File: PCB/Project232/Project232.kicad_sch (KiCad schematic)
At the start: 28 parts, among them J1 BOOT MODE, J2 USB_B_Micro, J3 SW, SW1 RESET, U1 STM32F103C8Tx, U2 AMS1117-3.3

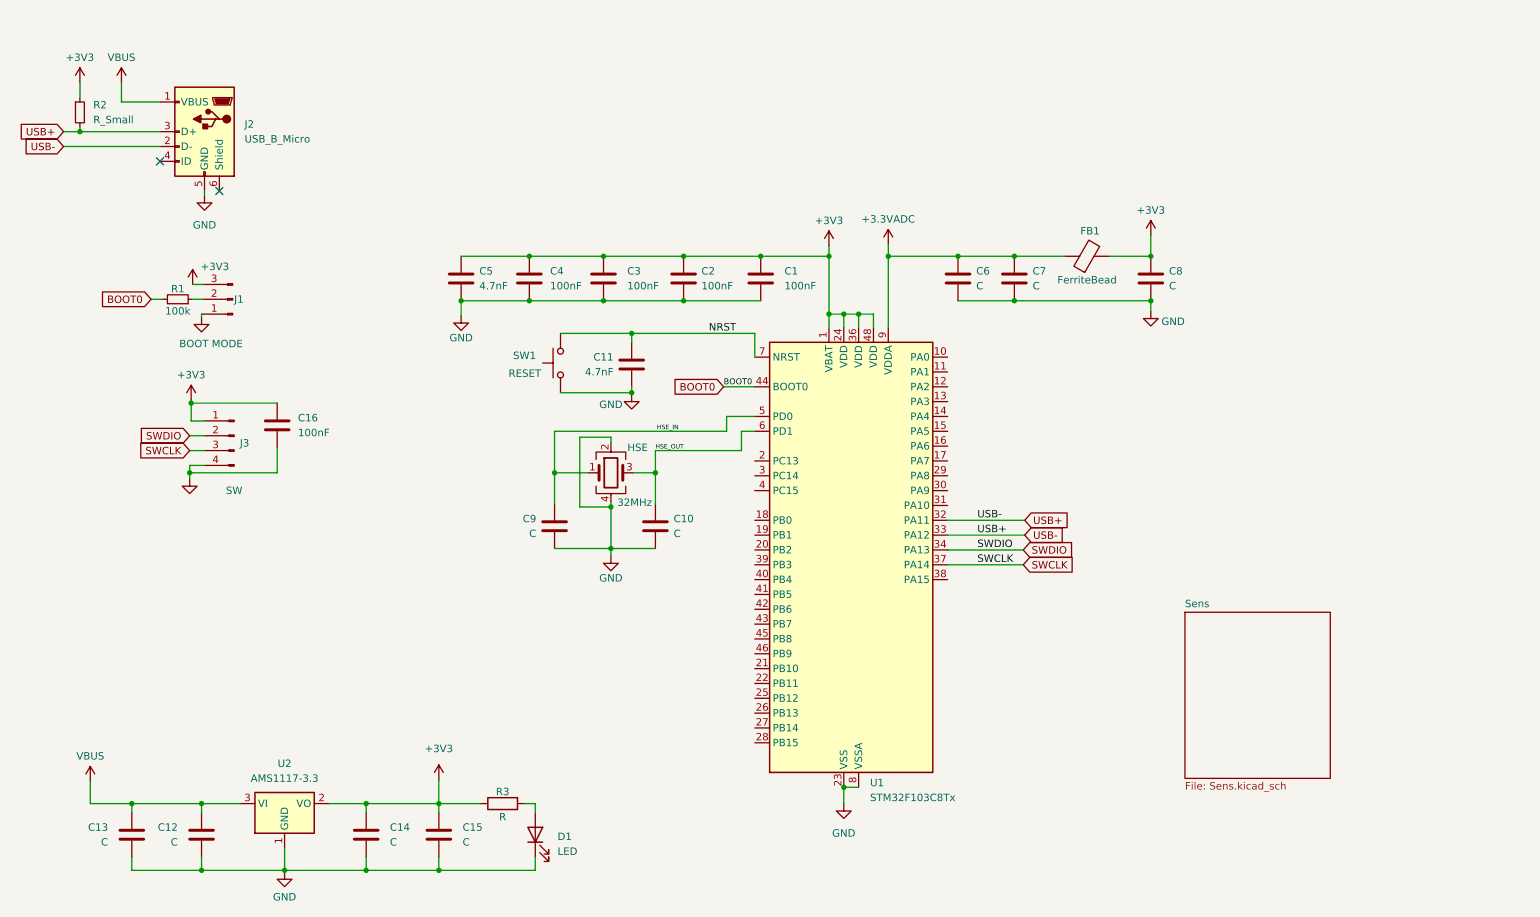
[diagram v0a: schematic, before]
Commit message: update test board and docs
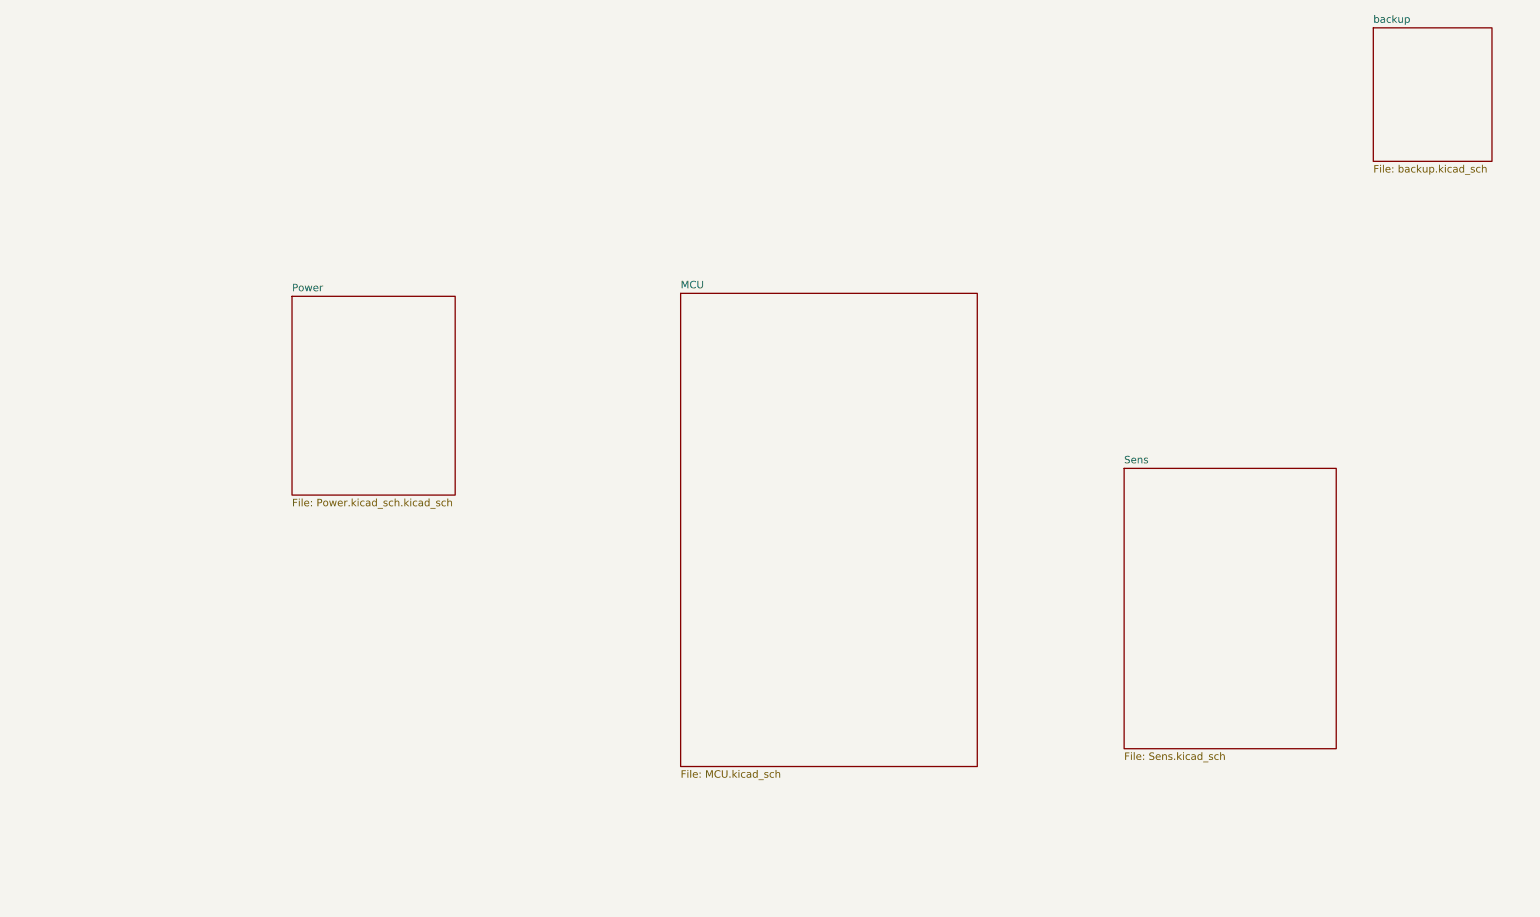
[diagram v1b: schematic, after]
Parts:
- removed C1, C16, C2, C3, C4: 100nF, symbol Device:C
- removed C10, C12, C13, C14, C15, C6, C7, C8, C9: C, symbol Device:C
- removed C11, C5: 4.7nF, symbol Device:C
- removed D1: LED, symbol Device:LED
- removed FB1: FerriteBead, symbol Device:FerriteBead
- removed HSE: 32MHz, symbol Device:Crystal_GND24
- removed J1: BOOT MODE, symbol Connector:Conn_01x03_Pin
- removed J2: USB_B_Micro, symbol Connector:USB_B_Micro
- removed J3: SW, symbol Connector:Conn_01x04_Pin
- removed R1: 100k, symbol Device:R_Small
- removed R2: R_Small, symbol Device:R_Small
- removed R3: R, symbol Device:R
- removed SW1: RESET, symbol Switch:SW_Push
- removed U1: STM32F103C8Tx, Package_QFP:LQFP-48_7x7mm_P0.5mm, symbol MCU_ST_STM32F1:STM32F103C8Tx
- removed U2: AMS1117-3.3, Package_TO_SOT_SMD:SOT-223-3_TabPin2, symbol Regulator_Linear:AMS1117-3.3
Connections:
- no-connect marks 2 -> 0
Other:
- added sheet MCU (MCU.kicad_sch)
- added sheet Power (Power.kicad_sch.kicad_sch)
- added sheet backup (backup.kicad_sch)
